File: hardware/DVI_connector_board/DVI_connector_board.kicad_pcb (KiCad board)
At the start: 2 copper layers, 18.6 x 22.9 mm, 6 parts, among them J1 FPC Cable connector 1x20, J2 HDMI

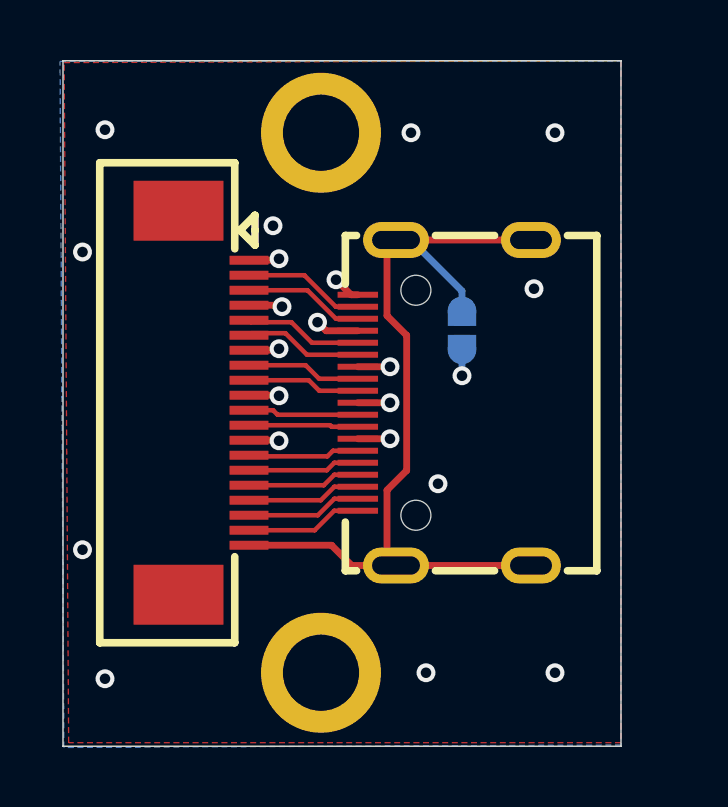
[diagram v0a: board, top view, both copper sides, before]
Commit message: update PCB design files
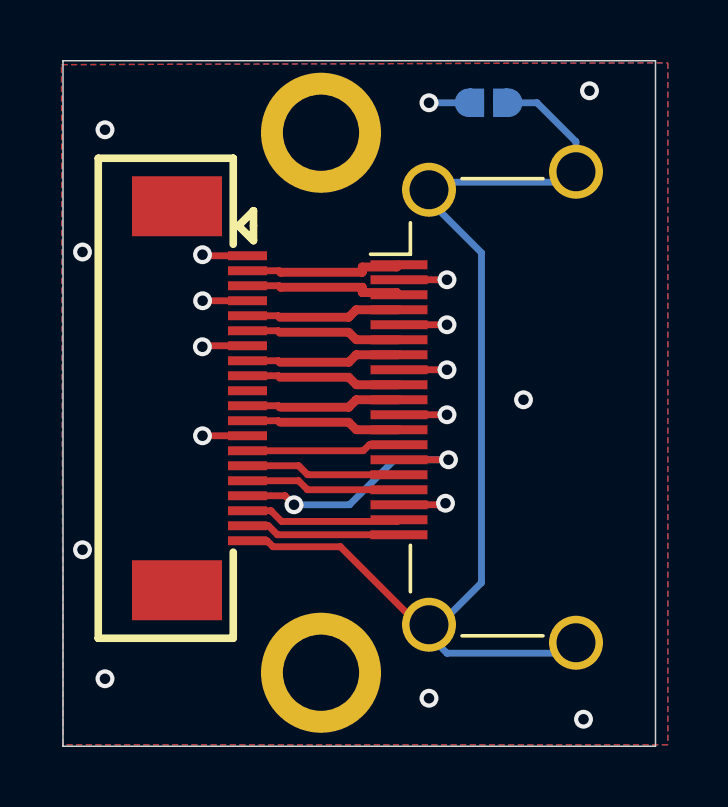
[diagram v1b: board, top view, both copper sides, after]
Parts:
- added G***: LOGO, LOGO, B.Cu at (113.8, 86.6)
- J2: value HDMI -> HDMI_A; footprint Library:Xunpu_HDMI-201 -> Connector_HDMI:HDMI_A_Amphenol_10029449-x01xLF_Horizontal
- moved JP1 7.64 mm to (121.6, 77.0), turned to 0 degrees
- moved J2 2.68 mm to (123.6, 87.2), turned to 90 degrees
- moved G*** 1.77 mm to (125.2, 87.5)
- moved J1 0.16 mm to (111.3, 86.8)
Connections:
- net Net-(J2-CK-) renamed /CK-
- net Net-(J2-D0-) renamed /D0-
- net Net-(J2-D1-) renamed /D1-
- net Net-(J2-D2-) renamed /D2-
- J1 pad 11: Net-(J2-CK+) -> /CK+
- J1 pad 2: Net-(J2-D2+) -> /D2+
- J1 pad 20: Net-(J2-SHELL) -> Net-(JP1-B)
- J1 pad 5: Net-(J2-D1+) -> /D1+
- J1 pad 8: Net-(J2-D0+) -> /D0+
- J2 pad 1: GND -> /D2+
- J2 pad 10: GND -> /CK+
- J2 pad 11: Net-(J2-CK+) -> GND
- J2 pad 13: GND -> Net-(J2-CEC)
- J2 pad 14: Net-(J2-CEC) -> Net-(J2-UTILITY)
- J2 pad 17: Net-(J2-UTILITY) -> GND
- J2 pad 2: Net-(J2-D2+) -> GND
- J2 pad 4: GND -> /D1+
- J2 pad 5: Net-(J2-D1+) -> GND
- J2 pad 7: GND -> /D0+
- J2 pad 8: Net-(J2-D0+) -> GND
- JP1 pad 2: Net-(J2-SHELL) -> Net-(JP1-B)
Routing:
- net Net-(JP1-B): track 0.00 -> 37.8 mm
- net Net-(J2-SHELL): track 29.5 -> 0.00 mm
- net Net-(J2-UTILITY): track 3.81 -> 9.10 mm, vias 0 -> 2
- net /D2+: track 0.00 -> 5.28 mm
- net /D1+: track 0.00 -> 5.17 mm
- net /CK+: track 0.00 -> 5.17 mm
- net /D0+: track 0.00 -> 5.17 mm
- net Net-(J2-D2+): track 4.06 -> 0.00 mm
- net Net-(J2-D1+): track 3.94 -> 0.00 mm
- net GND: track 11.7 -> 15.6 mm, vias 22 -> 18
- net Net-(J2-D0+): track 3.81 -> 0.00 mm
- net Net-(J2-CK+): track 3.69 -> 0.00 mm
- net /CK-: track 3.65 -> 5.17 mm
- net Net-(J2-SCL): track 3.73 -> 5.17 mm
- net Net-(J2-CEC): track 3.72 -> 5.13 mm
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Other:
- board size 18.6 x 22.9 mm -> 19.8 x 22.9 mm
- board text added: "2 layer JLC0216 1.6mm, 1oz coplanar 100 ohm differential width .2969mm, separation .2032mm"
